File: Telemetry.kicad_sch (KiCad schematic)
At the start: 0 parts

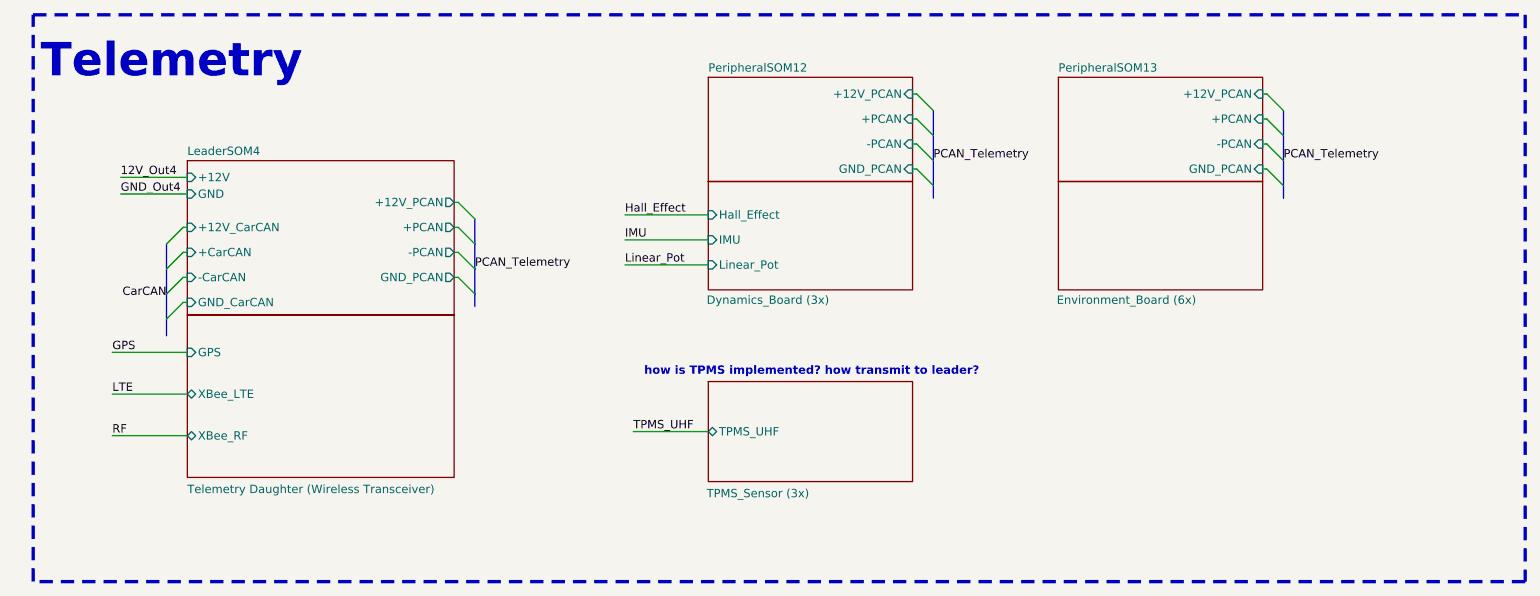
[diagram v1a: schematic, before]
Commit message: idk
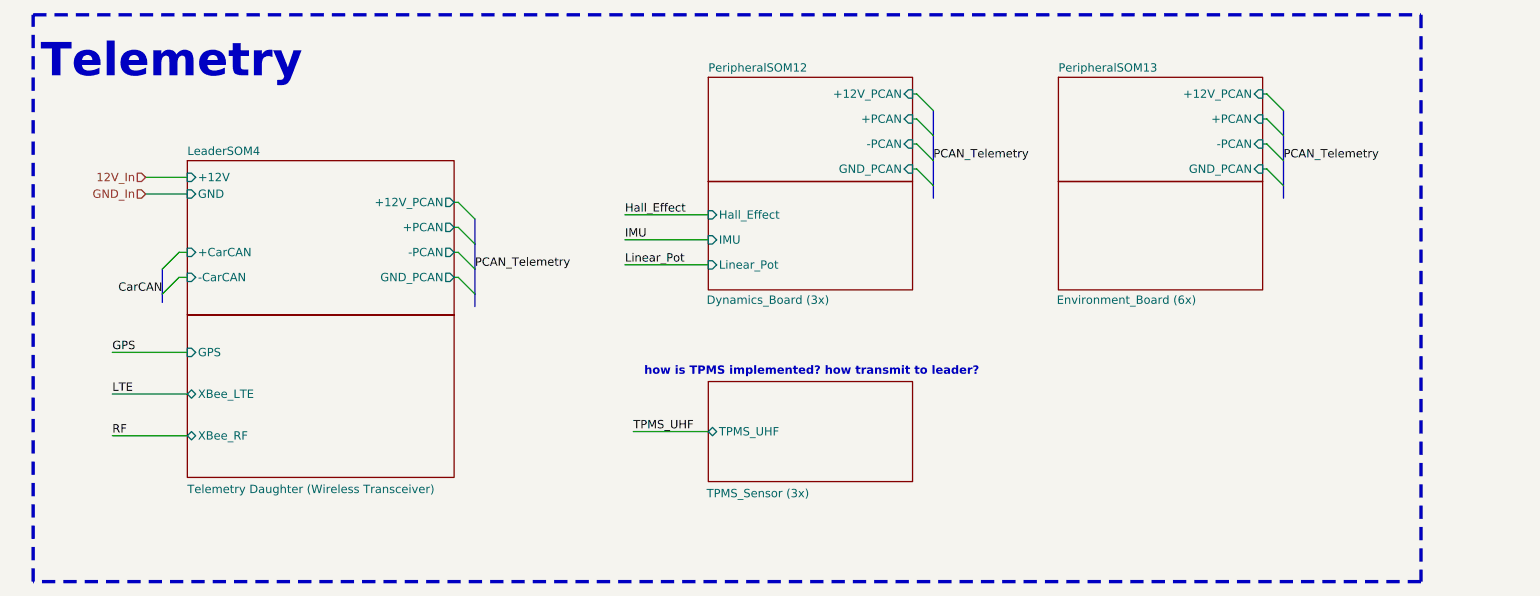
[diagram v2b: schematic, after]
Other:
- sheet LeaderSOM4 ports: added none; removed +12V_CarCAN, GND_CarCAN
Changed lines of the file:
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@@
 	(rectangle
 		(start 18.415 18.415)
-		(end 245.745 104.775)
+		(end 229.87 104.775)
 		(stroke
 			(width 0.508)
@@
 	)
 	(bus_entry
-		(at 38.735 60.96)
+		(at 38.1 60.96)
 		(size 2.54 -2.54)
 		(stroke
@@
 	)
 	(bus_entry
-		(at 38.735 57.15)
+		(at 38.1 57.15)
 		(size 2.54 -2.54)
 		(stroke
@@
 	)
 	(bus_entry
-		(at 38.735 53.34)
-		(size 2.54 -2.54)
-		(stroke
-			(width 0)
-			(type default)
-		)
-	)
-	(bus_entry
 		(at 153.035 34.29)
 		(size 2.54 2.54)
@@
 	)
 	(bus_entry
-		(at 38.735 64.77)
-		(size 2.54 -2.54)
-		(stroke
-			(width 0)
-			(type default)
-		)
-	)
-	(bus_entry
 		(at 206.375 30.48)
 		(size 2.54 2.54)
@@
 	(wire
 		(pts
+			(xy 40.64 58.42) (xy 41.91 58.42)
+		)
+		(stroke
+			(width 0)
+			(type default)
+		)
+	)
+	(wire
+		(pts
 			(xy 82.55 54.61) (xy 83.185 54.61)
 		)
@@
 	(bus
 		(pts
-			(xy 38.735 60.96) (xy 38.735 64.77)
-		)
-		(stroke
-			(width 0)
-			(type default)
-		)
-	)
-	(bus
-		(pts
 			(xy 85.725 57.15) (xy 85.725 60.96)
 		)
@@
 		)
 	)
-	(wire
-		(pts
-			(xy 41.275 54.61) (xy 41.91 54.61)
-		)
-		(stroke
-			(width 0)
-			(type default)
-		)
-	)
 	(bus
 		(pts
@@
 	(bus
 		(pts
-			(xy 38.735 57.15) (xy 38.735 60.96)
+			(xy 38.1 57.15) (xy 38.1 60.96)
 		)
 		(stroke
@@
 		(pts
 			(xy 108.585 52.705) (xy 121.285 52.705)
+		)
+		(stroke
+			(width 0)
+			(type default)
+		)
+	)
+	(wire
+		(pts
+			(xy 40.64 54.61) (xy 41.91 54.61)
 		)
 		(stroke
@@
 		)
 	)
+	(bus
+		(pts
+			(xy 38.1 60.96) (xy 38.1 62.23)
+		)
+		(stroke
+			(width 0)
+			(type default)
+		)
+	)
 	(wire
 		(pts
@@
 		(pts
 			(xy 82.55 50.8) (xy 83.185 50.8)
-		)
-		(stroke
-			(width 0)
-			(type default)
-		)
-	)
-	(wire
-		(pts
-			(xy 41.275 58.42) (xy 41.91 58.42)
 		)
 		(stroke
@@
 	(wire
 		(pts
-			(xy 41.275 50.8) (xy 41.91 50.8)
-		)
-		(stroke
-			(width 0)
-			(type default)
-		)
-	)
-	(bus
-		(pts
-			(xy 38.735 53.34) (xy 38.735 57.15)
-		)
-		(stroke
-			(width 0)
-			(type default)
-		)
-	)
-	(wire
-		(pts
-			(xy 41.275 62.23) (xy 41.91 62.23)
-		)
-		(stroke
-			(width 0)
-			(type default)
-		)
-	)
-	(wire
-		(pts
-			(xy 31.75 43.18) (xy 41.91 43.18)
+			(xy 35.56 43.18) (xy 41.91 43.18)
 		)
 		(stroke
@@
 		)
 	)
-	(bus
-		(pts
-			(xy 38.735 64.77) (xy 38.735 67.31)
-		)
-		(stroke
-			(width 0)
-			(type default)
-		)
-	)
 	(wire
 		(pts
@@
 	(wire
 		(pts
-			(xy 31.75 45.72) (xy 41.91 45.72)
+			(xy 35.56 45.72) (xy 41.91 45.72)
 		)
 		(stroke
@@
 		)
 	)
-	(label "12V_Out4"
-		(at 31.75 43.18 0)
-		(effects
-			(font
-				(size 1.27 1.27)
-			)
-			(justify left bottom)
-		)
-	)
 	(label "LTE"
 		(at 30.48 76.2 0)
@@
 	)
 	(label "CarCAN"
-		(at 38.735 61.595 180)
+		(at 38.1 60.96 180)
 		(effects
 			(font
@@
 		)
 	)
-	(label "GND_Out4"
-		(at 31.75 45.72 0)
-		(effects
-			(font
-				(size 1.27 1.27)
-			)
-			(justify left bottom)
-		)
-	)
 	(label "GPS"
 		(at 30.48 69.85 0)
@@
 			)
 			(justify left bottom)
+		)
+	)
+	(hierarchical_label "12V_In"
+		(shape input)
+		(at 35.56 43.18 180)
+		(effects
+			(font
+				(size 1.27 1.27)
+			)
+			(justify right)
+		)
+	)
+	(hierarchical_label "GND_In"
+		(shape input)
+		(at 35.56 45.72 180)
+		(effects
+			(font
+				(size 1.27 1.27)
+			)
+			(justify right)
 		)
 	)
@@
 			)
 		)
-		(pin "GND_CarCAN" input
-			(at 41.91 62.23 180)
-			(effects
-				(font
-					(size 1.27 1.27)
-				)
-				(justify left)
-			)
-		)
 		(pin "+12V_PCAN" output
 			(at 82.55 46.99 0)
@@
 			)
 		)
-		(pin "+12V_CarCAN" input
-			(at 41.91 50.8 180)
-			(effects
-				(font
-					(size 1.27 1.27)
-				)
-				(justify left)
-			)
-		)
